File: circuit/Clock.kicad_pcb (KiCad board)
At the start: 2 copper layers, 100 x 41 mm, 14 parts

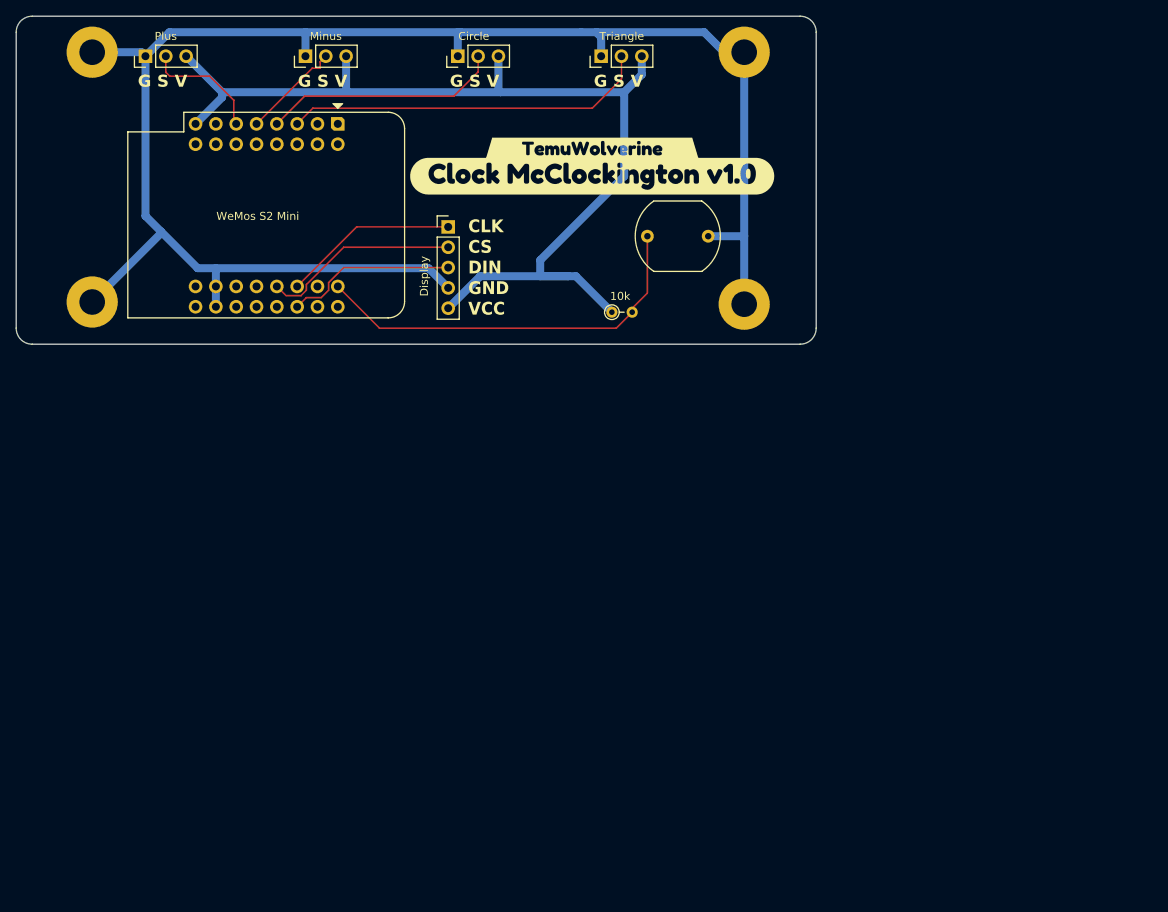
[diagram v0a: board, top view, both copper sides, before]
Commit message: updated to be gooderer
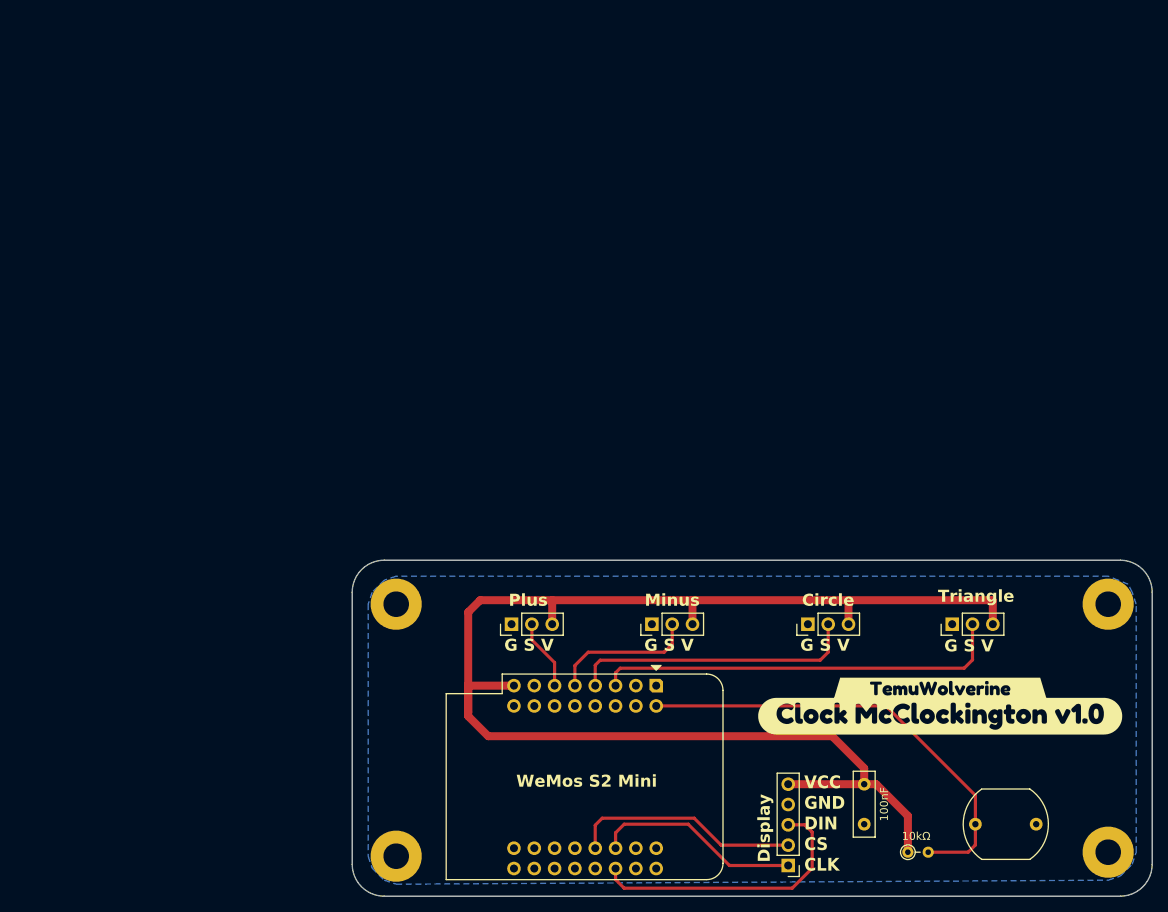
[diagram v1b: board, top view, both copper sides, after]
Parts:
- removed 10k: R, Resistor_THT:R_Axial_DIN0204_L3.6mm_D1.6mm_P2.54mm_Vertical
- removed WeMos S2 Mini: WeMos_S2_mini, wemos2:wemoss2
- added 100nF: 100nF, Capacitor_THT:C_Disc_D8.0mm_W2.5mm_P5.00mm, F.Cu at (129.5, 120.5)
- added 10kΩ: R, Resistor_THT:R_Axial_DIN0204_L3.6mm_D1.6mm_P2.54mm_Vertical, F.Cu at (135.0, 129.0)
- added U1: WeMos_S2_mini, wemos2:wemoss2, F.Cu at (103.5, 108.2)
- moved H3 161.6 mm to (160.0, 129.0)
- moved Display 90.4 mm to (120.0, 130.7), turned to 180 degrees
- moved Plus 84.5 mm to (85.4, 100.5)
- moved R2 84.2 mm to (143.4, 125.5)
- moved Triangle 83.5 mm to (140.5, 100.5)
- moved Circle 83.4 mm to (122.5, 100.5)
- moved Minus 83.2 mm to (103.0, 100.5)
- moved H1 82.7 mm to (160.0, 98.0)
- moved H2 81.6 mm to (71.0, 129.5)
- moved kibuzzard-696711A4 80.3 mm to (139.0, 108.5)
- moved kibuzzard-696745C6 80.3 mm to (139.0, 112.0)
- moved H4 53.6 mm to (71.0, 98.0)
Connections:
- net Net-(Circle1-Pin_3) renamed /Power
- Circle pad 2: Net-(Circle1-Pin_2) -> /CircleSignal
- Display pad 1: Net-(Display1-Pin_1) -> /Clock
- Display pad 2: Net-(Display1-Pin_2) -> /CS
- Display pad 3: Net-(Display1-Pin_3) -> /DisplaySignal
- Minus pad 2: Net-(Minus1-Pin_2) -> /MinusSignal
- Plus pad 2: Net-(Plus1-Pin_2) -> /PlusSignal
- R2 pad 1: Net-(U1-GPIO40) -> /PhotoresistorSignal
- Triangle pad 2: Net-(Triangle1-Pin_2) -> /TriangleSignal
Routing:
- net /Ground: track 208.8 -> 0.00 mm
- net /PhotoresistorSignal: track 0.00 -> 57.0 mm
- net /TriangleSignal: track 0.00 -> 51.4 mm
- net Net-(U1-GPIO40): track 50.1 -> 0.00 mm
- net Net-(Triangle1-Pin_2): track 45.7 -> 0.00 mm
- net /Power: track 131.4 -> 175.7 mm
- net /CircleSignal: track 0.00 -> 35.9 mm
- net /DisplaySignal: track 0.00 -> 35.3 mm
- net Net-(Circle1-Pin_2): track 29.8 -> 0.00 mm
- net /CS: track 0.00 -> 28.8 mm
- net /Clock: track 0.00 -> 26.1 mm
- net Net-(Display1-Pin_2): track 24.8 -> 0.00 mm
- net Net-(Display1-Pin_1): track 22.0 -> 0.00 mm
- net Net-(Display1-Pin_3): track 21.5 -> 0.00 mm
- net /MinusSignal: track 0.00 -> 18.3 mm
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- added copper zone on B.Cu, net /Ground
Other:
- board size 100 x 41 mm -> 100 x 42 mm
- board text added: "VCC GND DIN CS CLK"
- board text added: "WeMos S2 Mini"
- board text removed: "CLK CS DIN GND VCC"
